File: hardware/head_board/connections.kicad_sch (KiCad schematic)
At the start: 3 parts, among them J1 8P8C, J2 CAM, J6 CAMLED

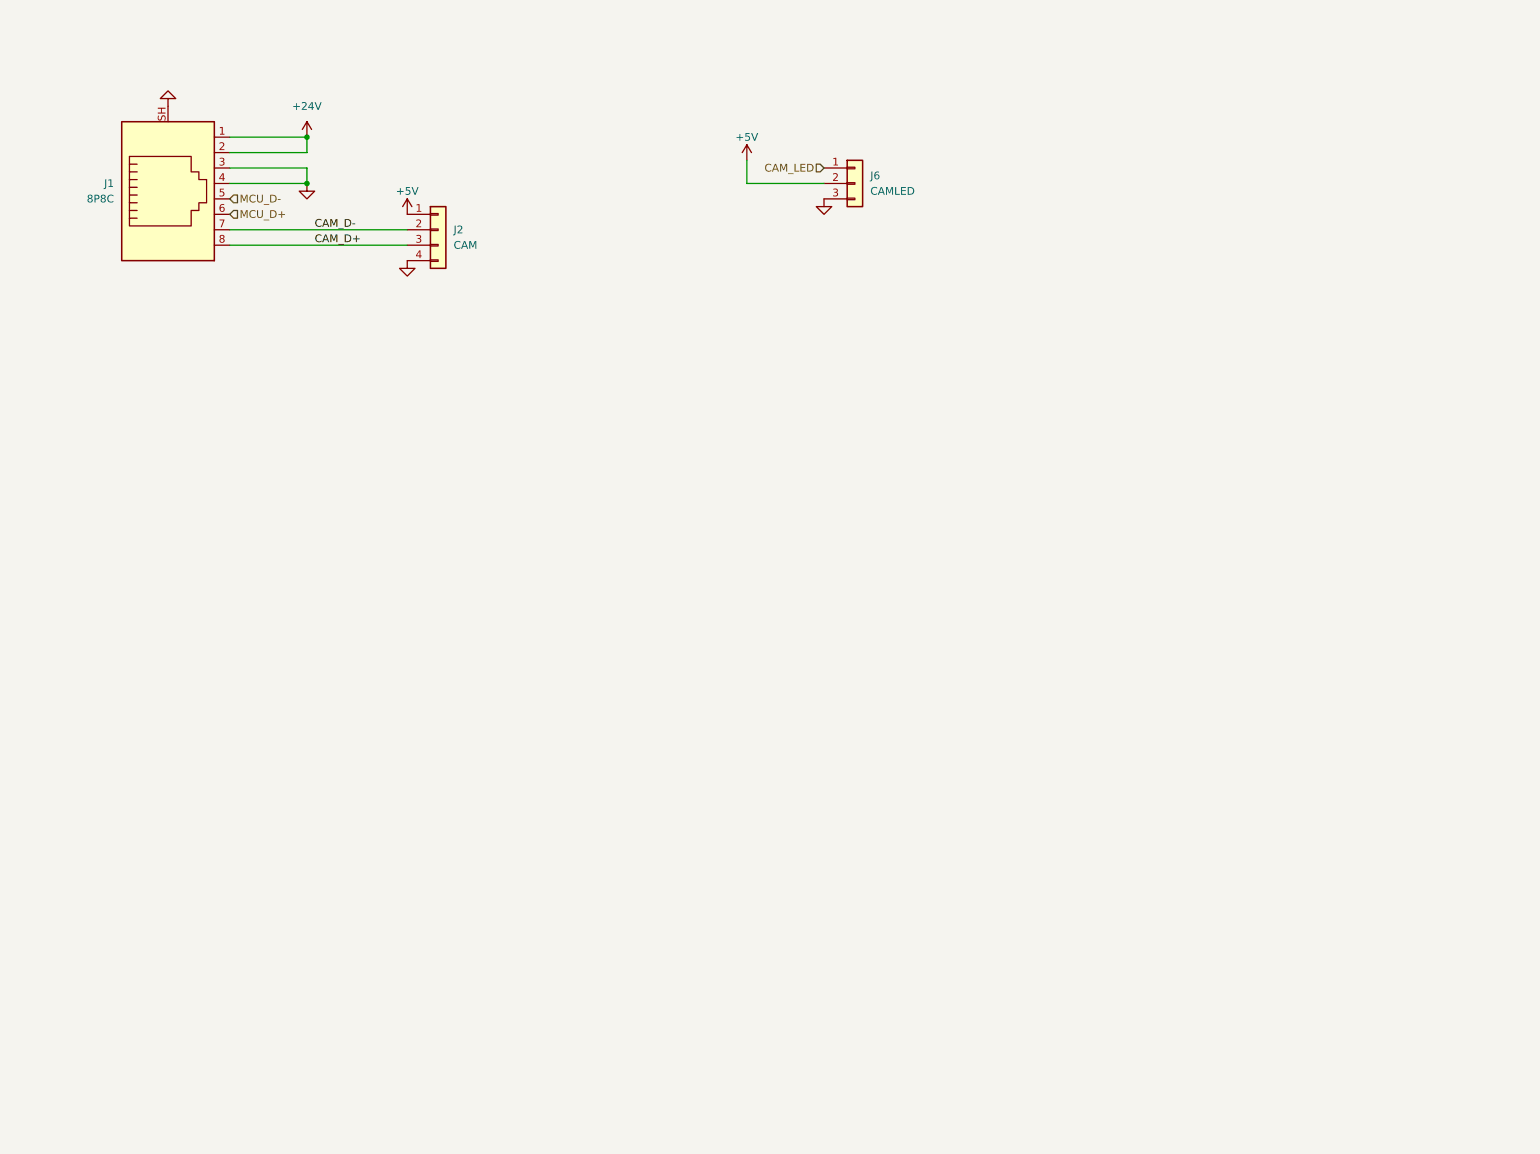
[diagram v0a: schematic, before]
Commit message: v1 revision to the schematic
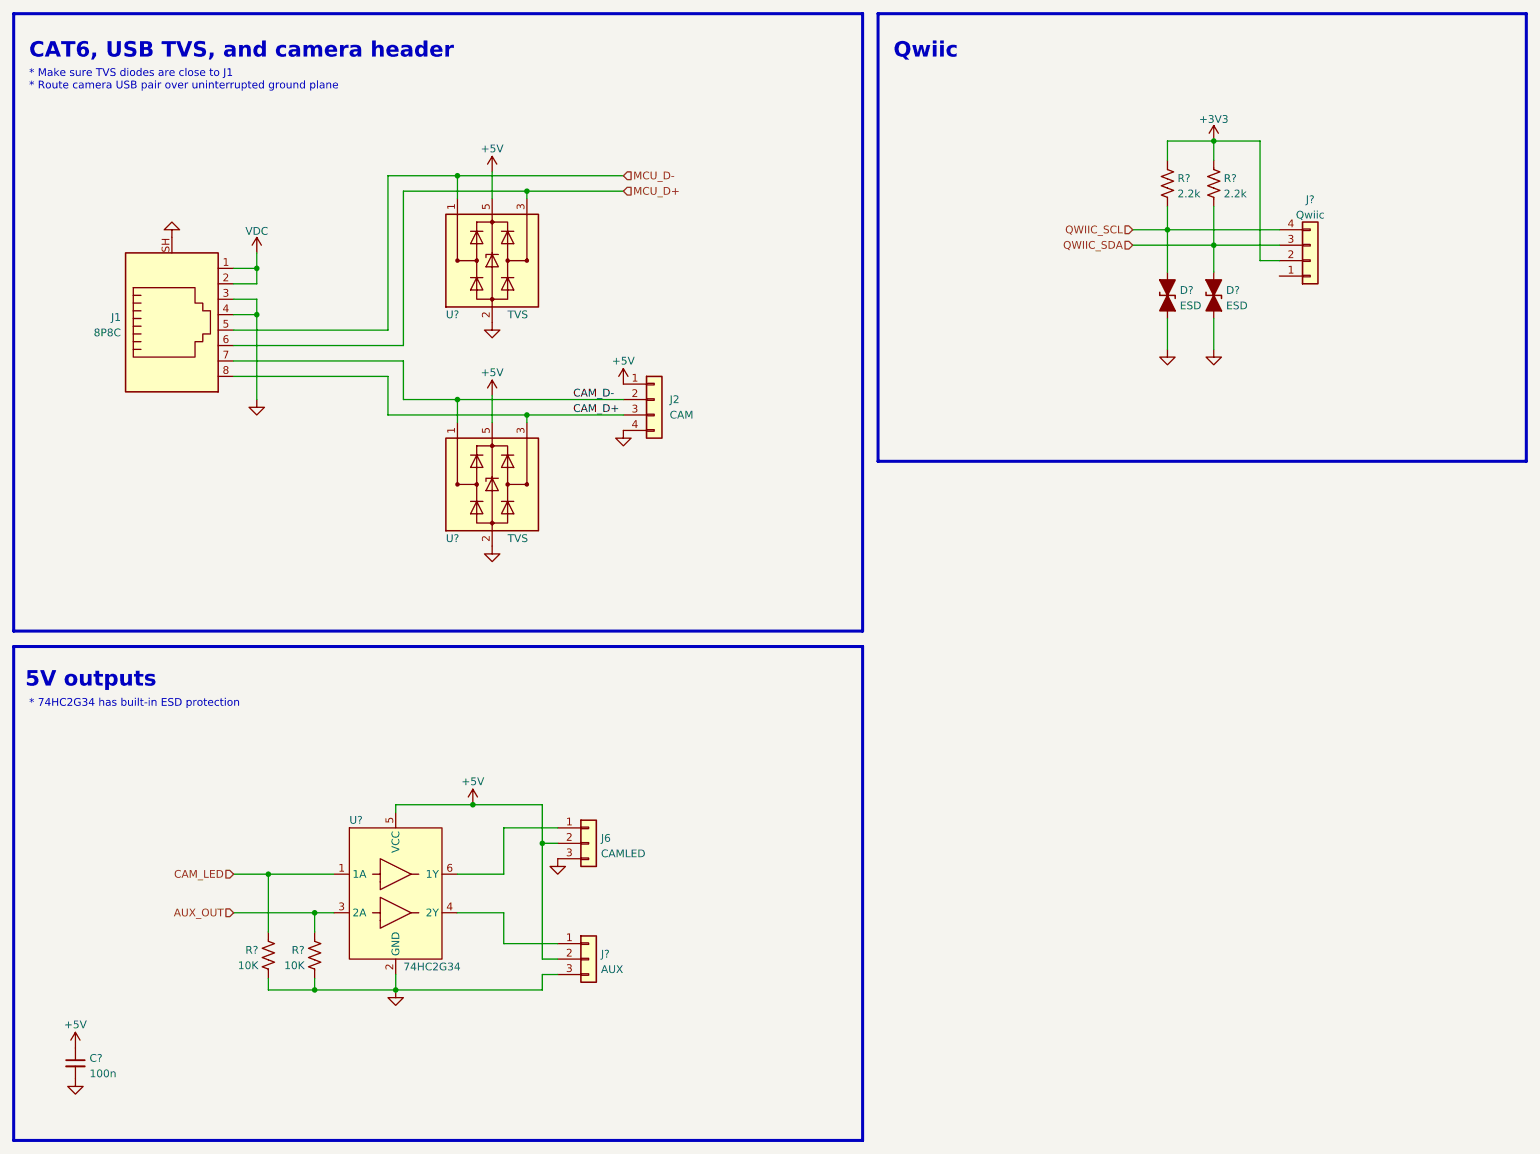
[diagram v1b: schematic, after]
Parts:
- added C?: 100n, Capacitor_SMD:C_0402_1005Metric_Pad0.74x0.62mm_HandSolder, symbol Device:C_Small
- added D? (x2): ESD, Capacitor_SMD:C_0603_1608Metric_Pad1.08x0.95mm_HandSolder, symbol Device:D_TVS_Filled
- added J?: Qwiic, Connector_JST:JST_PH_S4B-PH-SM4-TB_1x04-1MP_P2.00mm_Horizontal, symbol Connector_Generic:Conn_01x04
- added J?: AUX, Connector_JST:JST_XH_B3B-XH-AM_1x03_P2.50mm_Vertical, symbol Connector_Generic:Conn_01x03
- added R? (x2): 10K, Resistor_SMD:R_0402_1005Metric_Pad0.72x0.64mm_HandSolder, symbol Device:R_US
- added R? (x2): 2.2k, Resistor_SMD:R_0402_1005Metric_Pad0.72x0.64mm_HandSolder, symbol Device:R_US
- added U? (x2): TVS, Package_TO_SOT_SMD:SOT-23-6, symbol winterbloom:USBLC6-2SC6
- added U?: 74HC2G34, Package_TO_SOT_SMD:SOT-363_SC-70-6, symbol winterbloom:74HC2G34
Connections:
- net +5V: now also C?.1, J?.2 (Pin_2), U?.5 (VBUS), U?.5 (VBUS), U?.5 (VCC)
- net CAM_D+: now also U?.3 (D+), U?.4 (D+)
- net CAM_D-: now also U?.1 (D-), U?.6 (D-)
- net CAM_LED: now also R?.2, U?.1 (1A); no longer J6.1 (Pin_1)
- net GND: now also C?.2, D?.1 (A1), D?.1 (A1), J?.3 (Pin_3), R?.1, R?.1, U?.2 (GND), U?.2 (GND), U?.2 (GND)
- net MCU_D+: now also U?.3 (D+), U?.4 (D+)
- net MCU_D-: now also U?.1 (D-), U?.6 (D-)
- net +24V renamed VDC
- new net: J6.1 (Pin_1), U?.6 (1Y)
- new net: J?.1 (Pin_1), U?.4 (2Y)
- new net +3V3: J?.2 (Pin_2), R?.2, R?.2
- new net AUX_OUT: R?.2, U?.3 (2A)
- new net QWIIC_SCL: D?.2 (A2), J?.4 (Pin_4), R?.1
- new net QWIIC_SDA: D?.2 (A2), J?.3 (Pin_3), R?.1
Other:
- note added: "* 74HC2G34 has built-in ESD protection"
- note added: "* Make sure TVS diodes are close to J1 * Route camera USB pair over uninterrupted ground plane"
- note added: "5V outputs"
- note added: "CAT6, USB TVS, and camera header"
- note added: "Qwiic"
- company: (none) -> Winterbloom
- title: (none) -> Candela Head
- moved on the sheet: J1, J2, J6
